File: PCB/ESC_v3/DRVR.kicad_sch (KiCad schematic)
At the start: 18 parts, among them U2 DRV8323SRTAT

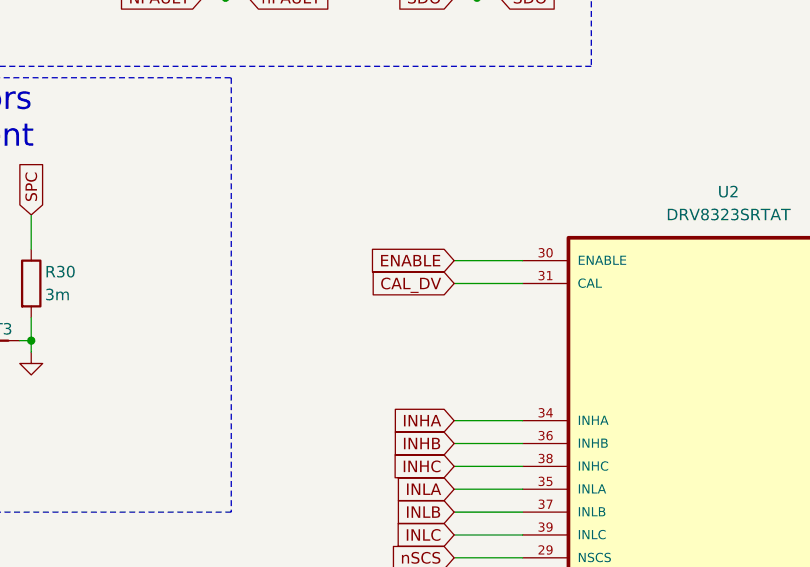
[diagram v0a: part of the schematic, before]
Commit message: Layout edit
Changed some layout and optimized
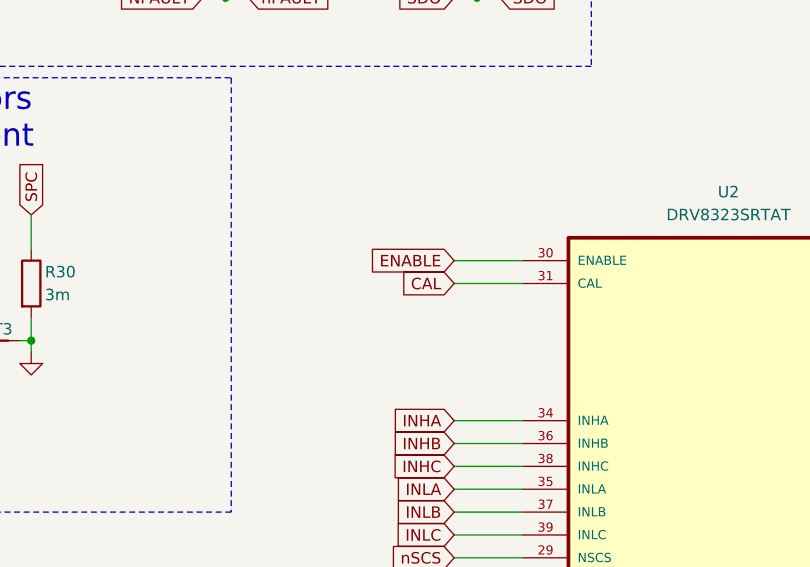
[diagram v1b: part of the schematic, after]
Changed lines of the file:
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@@
-		)
-	)
-	(global_label "CAL_DV"
-		(shape input)
-		(at 111.76 73.66 180)
-		(fields_autoplaced yes)
-		(effects
-			(font
-				(size 1.27 1.27)
-				(thickness 0.1588)
-			)
-			(justify right)
-		)
-		(property "Intersheetrefs" "${INTERSHEET_REFS}"
-			(at 101.5859 73.66 0)
-			(effects
-				(font
-					(size 1.27 1.27)
-				)
-				(justify right)
-				(hide yes)
-			)
 		)
 	)
@@
 			(effects
 				(font
+					(size 1.27 1.27)
+				)
+				(justify right)
+				(hide yes)
+			)
+		)
+	)
+	(global_label "CAL"
+		(shape input)
+		(at 111.76 73.66 180)
+		(fields_autoplaced yes)
+		(effects
+			(font
+				(size 1.27 1.27)
+				(thickness 0.1588)
+			)
+			(justify right)
+		)
+		(property "Intersheetrefs" "${INTERSHEET_REFS}"
+			(at 105.3881 73.66 0)
+			(effects
+				(font
